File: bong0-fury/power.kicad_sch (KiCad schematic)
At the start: 12 parts, among them J10 Eurorack_Power_10pin_Unshroud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, U1 TL072, U2 TL072, U3 TL072

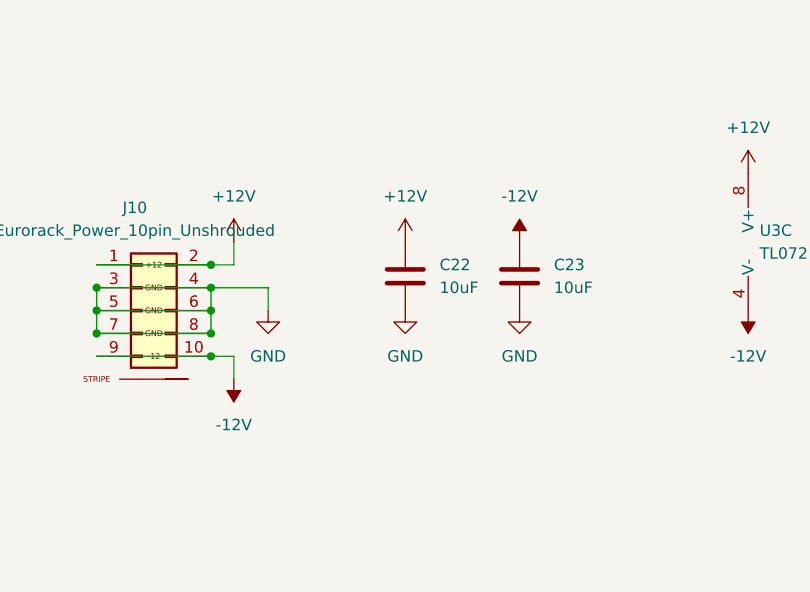
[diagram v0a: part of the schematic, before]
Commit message: Unknown changes
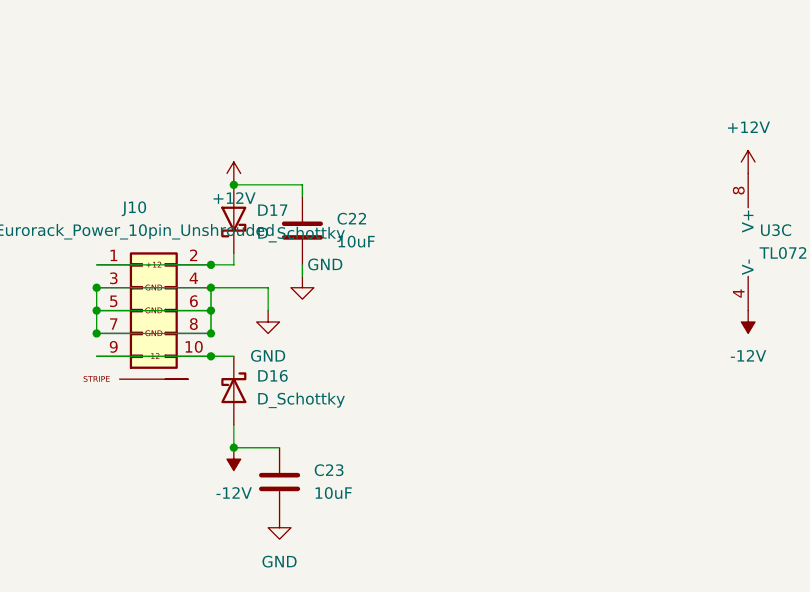
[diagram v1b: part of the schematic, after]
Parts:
- added D16, D17: D_Schottky, Diode_SMD:D_SOD-323, symbol Device:D_Schottky
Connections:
- net +12V: now also D17.2 (A); no longer J10.1 (+12V), J10.2 (+12V)
- net -12V: now also D16.2 (A); no longer J10.10 (-12V), J10.9 (-12V)
- new net: D17.1 (K), J10.1 (+12V), J10.2 (+12V)
- new net: D16.1 (K), J10.10 (-12V), J10.9 (-12V)
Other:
- moved on the sheet: C22, C23
